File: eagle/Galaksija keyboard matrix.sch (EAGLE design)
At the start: 63 parts

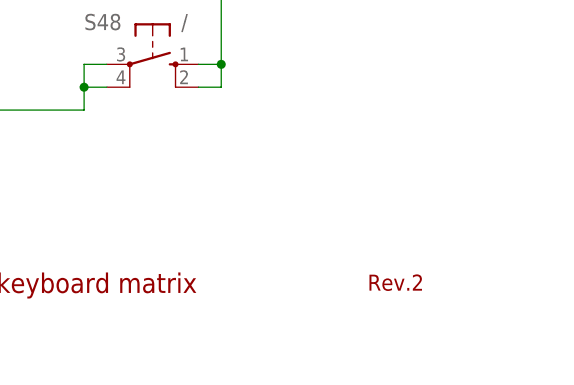
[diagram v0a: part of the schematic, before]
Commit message: finished keyboard revision 3
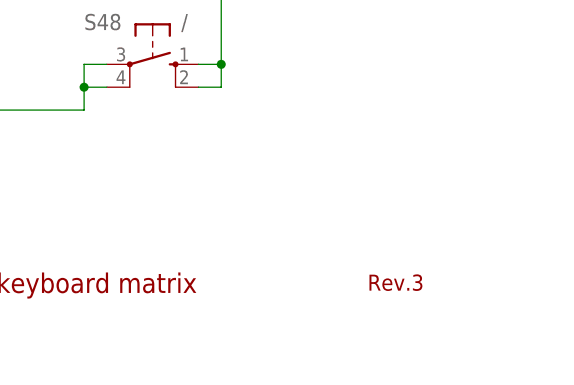
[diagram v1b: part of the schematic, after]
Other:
- note added: "Rev.3"
- note removed: "Rev.2"
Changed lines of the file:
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@@
 <plain>
 <text x="78.74" y="-40.64" size="2.1844" layer="94">Galaksija keyboard matrix</text>
-<text x="133.096" y="-40.386" size="1.778" layer="94">Rev.2</text>
+<text x="133.096" y="-40.386" size="1.778" layer="94">Rev.3</text>
 </plain>
 <instances>
